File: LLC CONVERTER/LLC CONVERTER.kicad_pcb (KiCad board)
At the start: 2 copper layers, 1 part, among them IC1 UCC256601DDBR

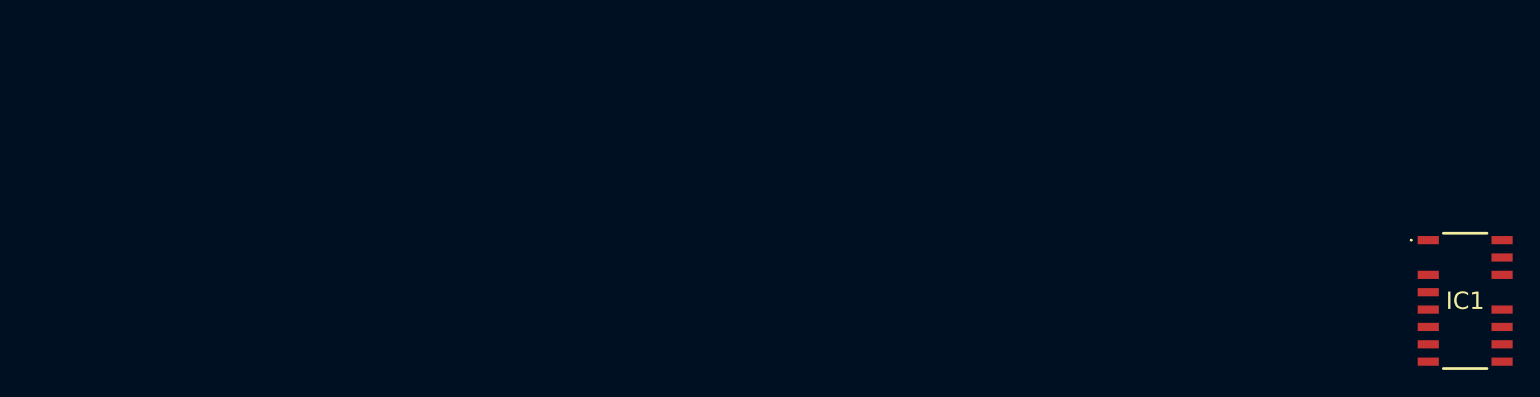
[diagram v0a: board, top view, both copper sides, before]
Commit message: change kiya
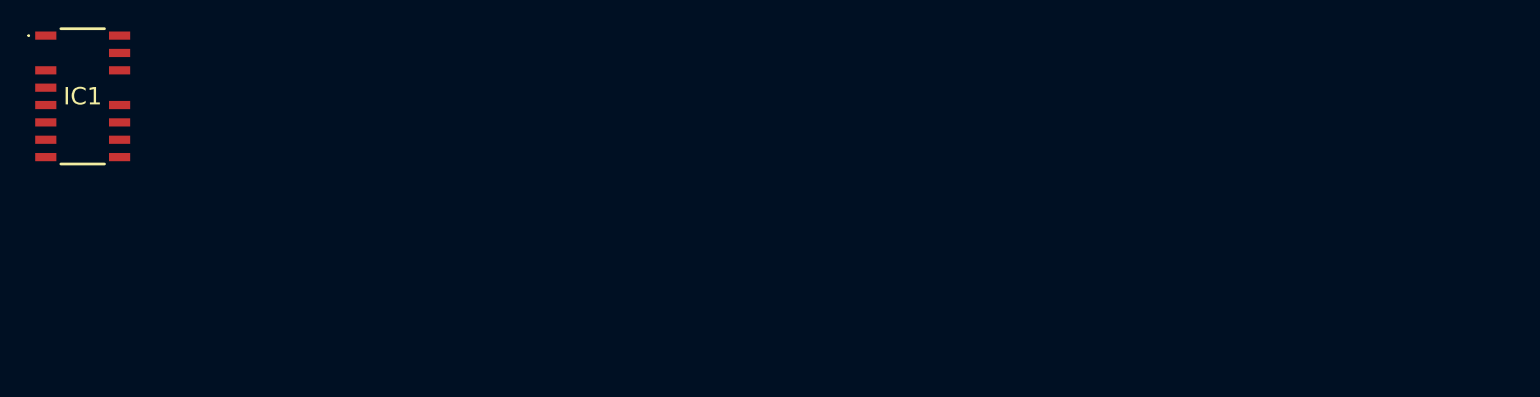
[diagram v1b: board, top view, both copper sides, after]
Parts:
- moved IC1 102.3 mm to (71.9, 69.8)
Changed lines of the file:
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@@
 	(footprint "PCB:UCC256601DDBR"
 		(layer "F.Cu")
-		(at 173.05 84.745)
+		(at 71.9 69.78)
 		(descr "UCC256601DDBR-2")
 		(tags "Integrated Circuit")
